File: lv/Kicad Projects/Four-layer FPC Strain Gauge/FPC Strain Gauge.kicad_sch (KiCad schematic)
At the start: 20 parts, among them J1 Conn_01x04, U1 INA333xxDGK, U2 OPA333xxDBV

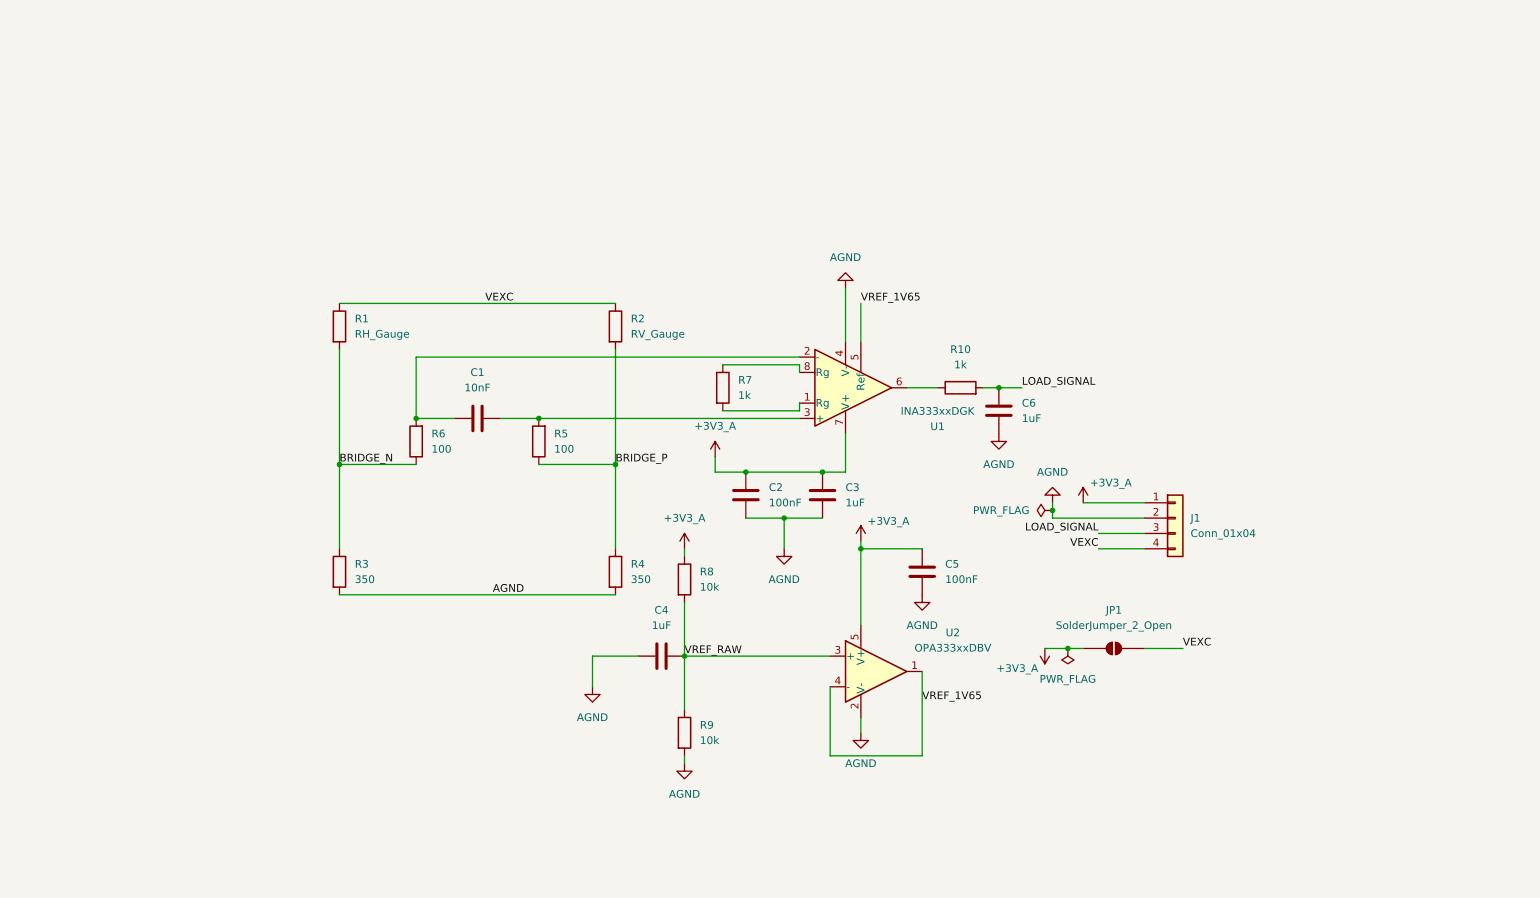
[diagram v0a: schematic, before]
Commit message: Finish Schematic
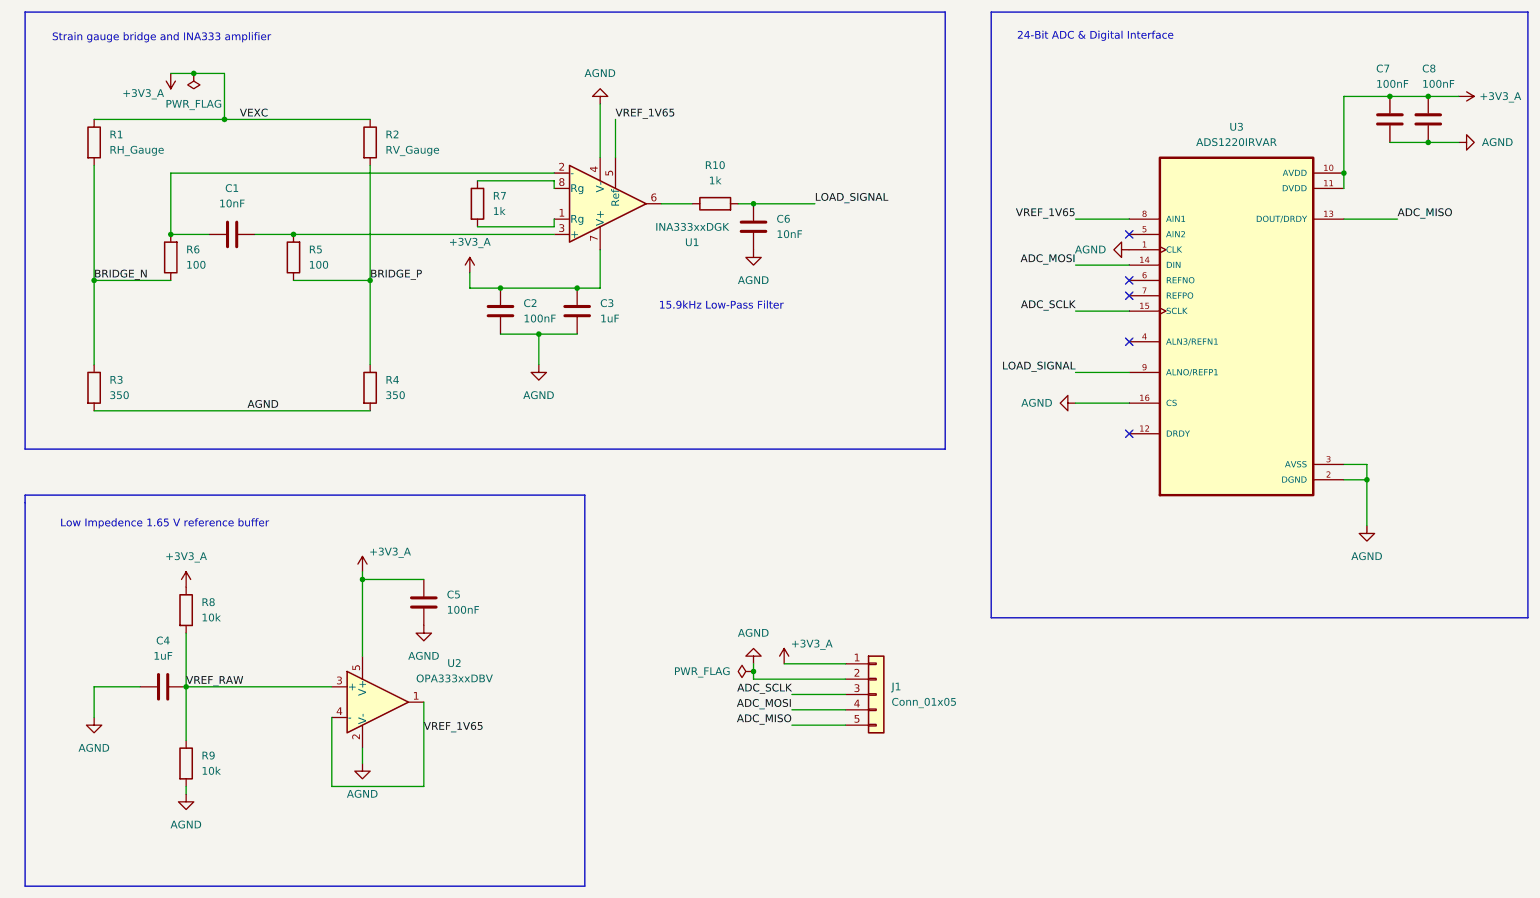
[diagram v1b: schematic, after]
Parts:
- removed J1: Conn_01x04, Package_DFN_QFN:WDFN-10-1EP_3x3mm_P0.5mm_EP1.8x2.5mm, symbol Connector_Generic:Conn_01x04
- removed JP1: SolderJumper_2_Open, symbol Jumper:SolderJumper_2_Open
- added C7, C8: 100nF, symbol Device:C
- added J1: Conn_01x05, Connector_Audio:Jack_XLR_Neutrik_NC3FAAH_Horizontal, symbol Connector_Generic:Conn_01x05
- added U3: ADS1220IRVAR, ADS1220IRVAR:QFN50P350X350X100-17N, symbol ADS1220IRVAR:ADS1220IRVAR
- C6: value 1uF -> 10nF
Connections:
- net VEXC is gone; now on net +3V3_A: R1.1, R2.1
- net +3V3_A: now also C7.1, C8.1, J1.1 (Pin_1), U3.10 (AVDD), U3.11 (DVDD)
- net AGND: now also C7.2, C8.2, J1.2 (Pin_2), U3.1 (CLK), U3.16 (CS), U3.2 (DGND), U3.3 (AVSS)
- net LOAD_SIGNAL: now also U3.9 (ALNO/REFP1)
- net VREF_1V65: now also U3.8 (AIN1)
- new net ADC_MISO: J1.5 (Pin_5), U3.13 (DOUT/DRDY)
- new net ADC_MOSI: J1.4 (Pin_4), U3.14 (DIN)
- new net ADC_SCLK: J1.3 (Pin_3), U3.15 (SCLK)
- no-connect marks 0 -> 5
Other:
- note added: "15.9kHz Low-Pass Filter"
- note added: "24-Bit ADC & Digital Interface"
- note added: "Low Impedence 1.65 V reference buffer"
- note added: "Strain gauge bridge and INA333 amplifier"
- title: ${BOARD_TITLE} -> FPC Strain Guage + Instrumentation
- moved on the sheet: C1, C2, C3, C4, C5, C6, R1, R10, R2, R3, R4, R5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
